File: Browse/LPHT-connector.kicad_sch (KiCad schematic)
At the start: 6 parts, among them J7 LPHT-04-16-L-RT1-GP

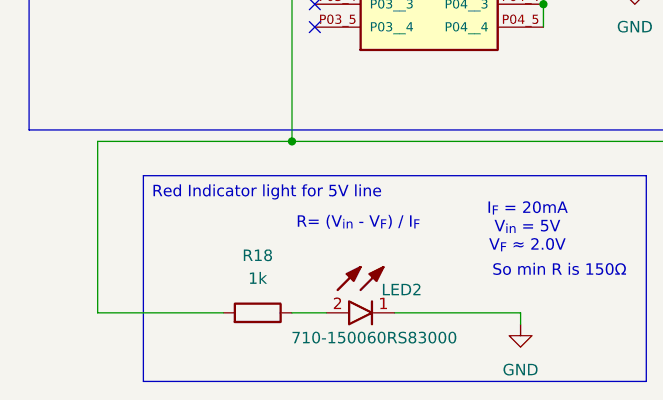
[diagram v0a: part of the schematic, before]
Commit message: Deploying to gh-pages from @ Nautilus-UUV/nautilus-mainboard-PCB@2b5265db7706a31505c0a0411337a4a604b5fb21 🚀
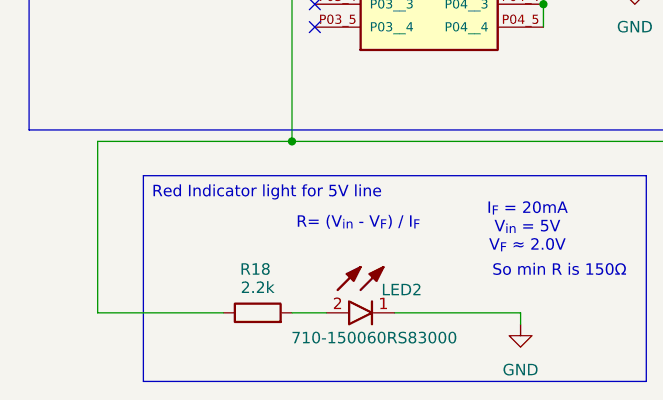
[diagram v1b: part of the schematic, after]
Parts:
- removed R18: 1k, Resistor_SMD:R_0603_1608Metric, symbol #dzdb:g_res/R-1k-0603
- added R18: 2.2k, Resistor_SMD:R_0603_1608Metric, symbol #dzdb:g_res/R-2.2k-0603
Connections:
- net Battery_Out_5V: now also R18.1
- net at LED2.2 (A): now also R18.2
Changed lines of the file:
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@@
+    )
+  )
+  (symbol (lib_id "#dzdb:g_res/R-2.2k-0603") (at 134.62 162.56 90) (unit 1)
+    (exclude_from_sim no) (in_bom yes) (on_board yes) (dnp no)
+    (property "Reference" "R18" (at 134.366 157.734 90)
+      (effects (font (size 1.27 1.27)))
+    )
+    (property "Value" "2.2k" (at 134.62 159.766 90)
+      (effects (font (size 1.27 1.27)))
+    )
+    (property "Footprint" "Resistor_SMD:R_0603_1608Metric" (at 134.62 164.338 90)
+      (effects (font (size 1.27 1.27)) (hide yes))
+    )
+    (property "Datasheet" "https://www.we-online.com/components/products/datasheet/560112116098.pdf" (at 134.62 162.56 0)
+      (effects (font (size 1.27 1.27)) (hide yes))
+    )
+    (property "Description" "Thick Film Resistors - SMD WRIS-RSKS 2.2 kOhms 1 % 0.1 W 0603" (at 134.62 162.56 0)
+      (effects (font (size 1.27 1.27)) (hide yes))
+    )
+    (property "IPN" "R-2.2k-0603" (at 134.62 162.56 0)
+      (effects (font (size 1.27 1.27)) (hide yes))
+    )
+    (property "MPN" "560112116098" (at 134.62 162.56 0)
+      (effects (font (size 1.27 1.27)) (hide yes))
+    )
+    (property "Manufacturer" "Wurth Elektronik" (at 134.62 162.56 0)
+      (effects (font (size 1.27 1.27)) (hide yes))
+    )
+    (property "Resistance" "2.2k" (at 134.62 162.56 0)
+      (effects (font (size 1.27 1.27)) (hide yes))
+    )
+    (property "Power" "0.1 W" (at 134.62 162.56 0)
+      (effects (font (size 1.27 1.27)) (hide yes))
+    )
+    (property "Material" "Thick film" (at 134.62 162.56 0)
+      (effects (font (size 1.27 1.27)) (hide yes))
+    )
+    (property "Tolerance" "1 %" (at 134.62 162.56 0)
+      (effects (font (size 1.27 1.27)) (hide yes))
+    )
+    (property "Supplier" "Mouser" (at 134.62 162.56 0)
+      (effects (font (size 1.27 1.27)) (hide yes))
+    )
+    (property "SPN" "710-560112116098" (at 134.62 162.56 0)
+      (effects (font (size 1.27 1.27)) (hide yes))
+    )
+    (property "LCSC" "CXXXXX" (at 134.62 162.56 0)
+      (effects (font (size 1.27 1.27)) (hide yes))
+    )
+    (property "Comment" "lifecycle=Active; note=Auto-generated" (at 134.62 162.56 0)
+      (effects (font (size 1.27 1.27)) (hide yes))
+    )
+    (pin "1")
+    (pin "2")
+    (instances
+      (project ""
+        (path "/ce1819b2-f280-40ed-834f-6fe4d12f809d/8ca810bd-6311-4873-a4c4-10e0b1989f7a"
+          (reference "R18") (unit 1)
+        )
+      )
     )
   )
@@
         )
       )
-    )
-  )
-  (symbol (lib_id "#dzdb:g_res/R-1k-0603") (at 134.62 162.56 270) (mirror x) (unit 1)
-    (exclude_from_sim no) (in_bom yes) (on_board yes) (dnp no) (fields_autoplaced)
-    (property "Reference" "R18" (at 134.62 156.21 90)
-      (effects (font (size 1.27 1.27)))
-    )
-    (property "Value" "1k" (at 134.62 158.75 90)
-      (effects (font (size 1.27 1.27)))
-    )
-    (property "Footprint" "Resistor_SMD:R_0603_1608Metric" (at 134.62 164.338 90)
-      (effects (font (size 1.27 1.27)) (hide yes))
-    )
-    (property "Datasheet" "https://www.we-online.com/components/products/datasheet/560112116014.pdf" (at 134.62 162.56 0)
-      (effects (font (size 1.27 1.27)) (hide yes))
-    )
-    (property "Description" "Thick Film Resistors - SMD WRIS-RSKS 1 kOhms 1 % 0.1 W 0603" (at 134.62 162.56 0)
-      (effects (font (size 1.27 1.27)) (hide yes))
-    )
-    (property "IPN" "R-1k-0603" (at 134.62 162.56 0)
-      (effects (font (size 1.27 1.27)) (hide yes))
-    )
-    (property "MPN" "560112116014" (at 134.62 162.56 0)
-      (effects (font (size 1.27 1.27)) (hide yes))
-    )
-    (property "Manufacturer" "Wurth Elektronik" (at 134.62 162.56 0)
-      (effects (font (size 1.27 1.27)) (hide yes))
-    )
-    (property "Resistance" "1k" (at 134.62 162.56 0)
-      (effects (font (size 1.27 1.27)) (hide yes))
-    )
-    (property "Power" "0.1 W" (at 134.62 162.56 0)
-      (effects (font (size 1.27 1.27)) (hide yes))
-    )
-    (property "Material" "Thick film" (at 134.62 162.56 0)
-      (effects (font (size 1.27 1.27)) (hide yes))
-    )
-    (property "Tolerance" "1 %" (at 134.62 162.56 0)
-      (effects (font (size 1.27 1.27)) (hide yes))
-    )
-    (property "Supplier" "Mouser" (at 134.62 162.56 0)
-      (effects (font (size 1.27 1.27)) (hide yes))
-    )
-    (property "SPN" "710-560112116014" (at 134.62 162.56 0)
-      (effects (font (size 1.27 1.27)) (hide yes))
-    )
-    (property "LCSC" "CXXXXX" (at 134.62 162.56 0)
-      (effects (font (size 1.27 1.27)) (hide yes))
-    )
-    (property "Comment" "lifecycle=Active; note=Auto-generated" (at 134.62 162.56 0)
-      (effects (font (size 1.27 1.27)) (hide yes))
-    )
-    (pin "1")
-    (pin "2")
-    (instances
-      (project "nautilus_mainboard"
-        (path "/ce1819b2-f280-40ed-834f-6fe4d12f809d/8ca810bd-6311-4873-a4c4-10e0b1989f7a"
-          (reference "R18") (unit 1)
-        )
-      )
